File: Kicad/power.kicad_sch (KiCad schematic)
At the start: 24 parts, among them CN1 XT30PW-M, J5 Ext. bulk, U7 LMR51610XDBVR, U8 TLV75733PDBV

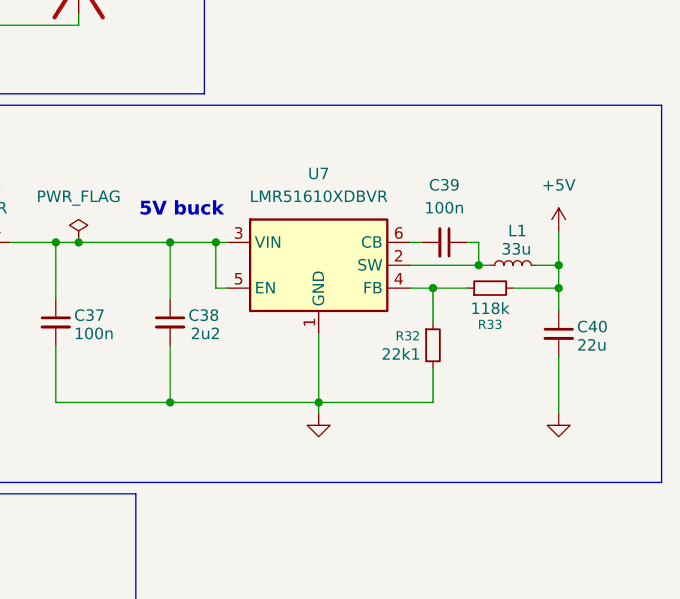
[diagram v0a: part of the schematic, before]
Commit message: commit
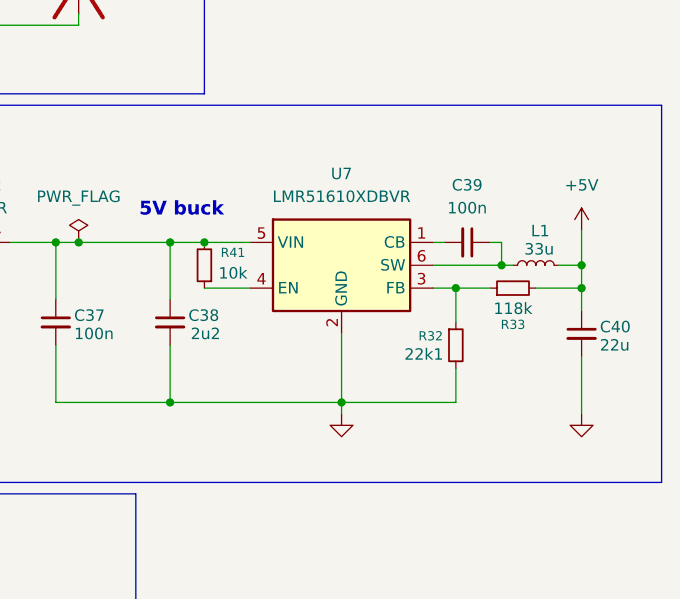
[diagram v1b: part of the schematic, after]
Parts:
- added R41: 10k, Resistor_SMD:R_0402_1005Metric, symbol Device:R_Small
- J5: footprint addons:2p WireSolder 1.5mmID_2.5mmOD -> addons:2p WireSolder 1.3mmID_2mmOD
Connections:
- net GND: now also U7.2 (GND); no longer U7.1 (GND)
- net at C39.1, L1.1: now also U7.6 (SW); no longer U7.2 (SW)
- net at C39.2: now also U7.1 (CB); no longer U7.6 (CB)
- net at C37.1, C38.1, FB2.2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: now also R41.2; no longer U7.3 (VIN)
- net at R32.1, R33.1: now also U7.3 (FB); no longer U7.4 (FB)
- new net: R41.1, U7.4 (EN)
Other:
- moved on the sheet: C39, C40, L1, R32, R33, U7
